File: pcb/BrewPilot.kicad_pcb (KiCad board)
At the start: 2 copper layers, 113 x 129 mm, 57 parts, among them J1 5V Power, J10 Boiler Probe, J11 SOL_L_FUSE, J12 5V_FUSE_5x20mm, J13 I2C Port, J2 Flow Meter Group One, J3 Flow Meter Group Two, J4 FlexGPIO_1, J5 FlexGPIO_2, J6 RelayOut_1, J7 RelayOut2, J8 Solenoid Power, J9 Pump Power, K1 G3MB-202P DC5, K2 G3MB-202P DC5, K3 G3MB-202P DC5, K4 G3MB-202P DC5, K5 G3MB-202P DC5, Q1 BC547, Q2 BC547, Q3 BC547, Q4 BC547, Q5 BC547, U1 esp32

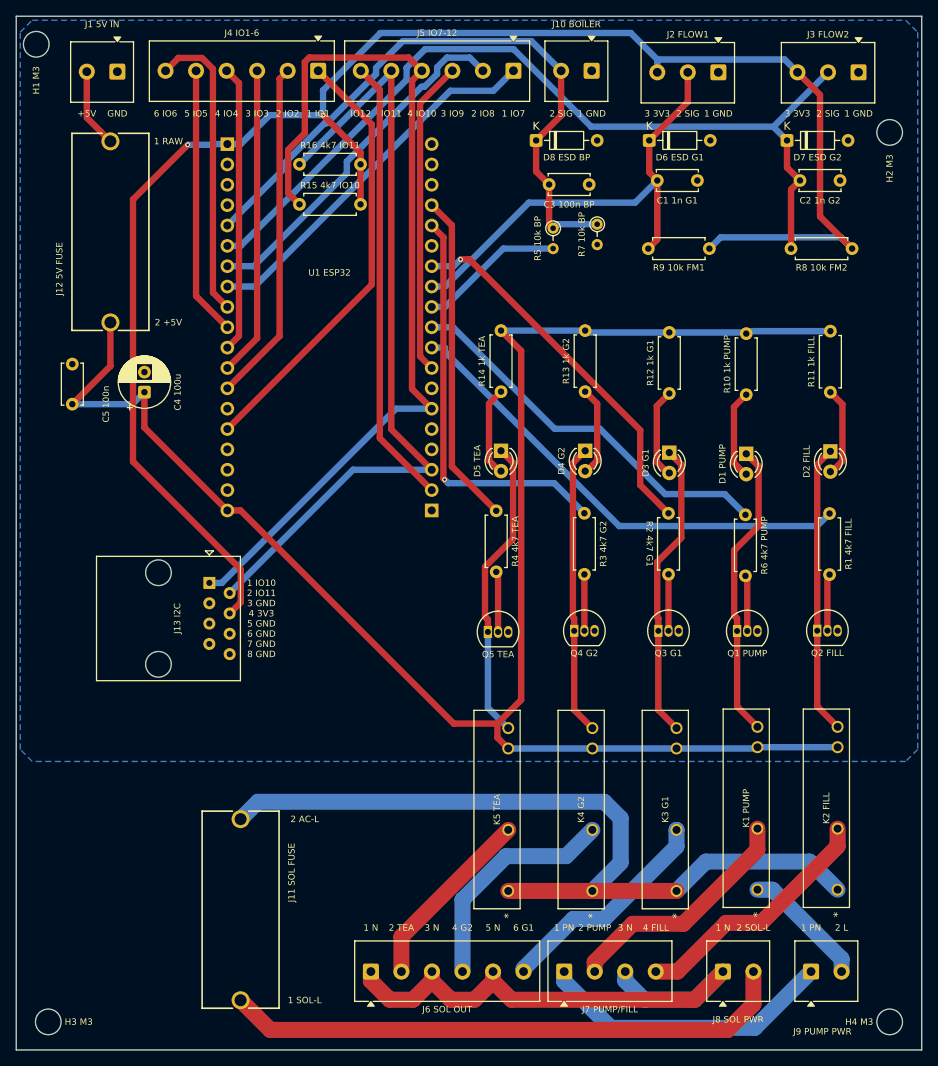
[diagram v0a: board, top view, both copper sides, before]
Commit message: made pcb layout more compact
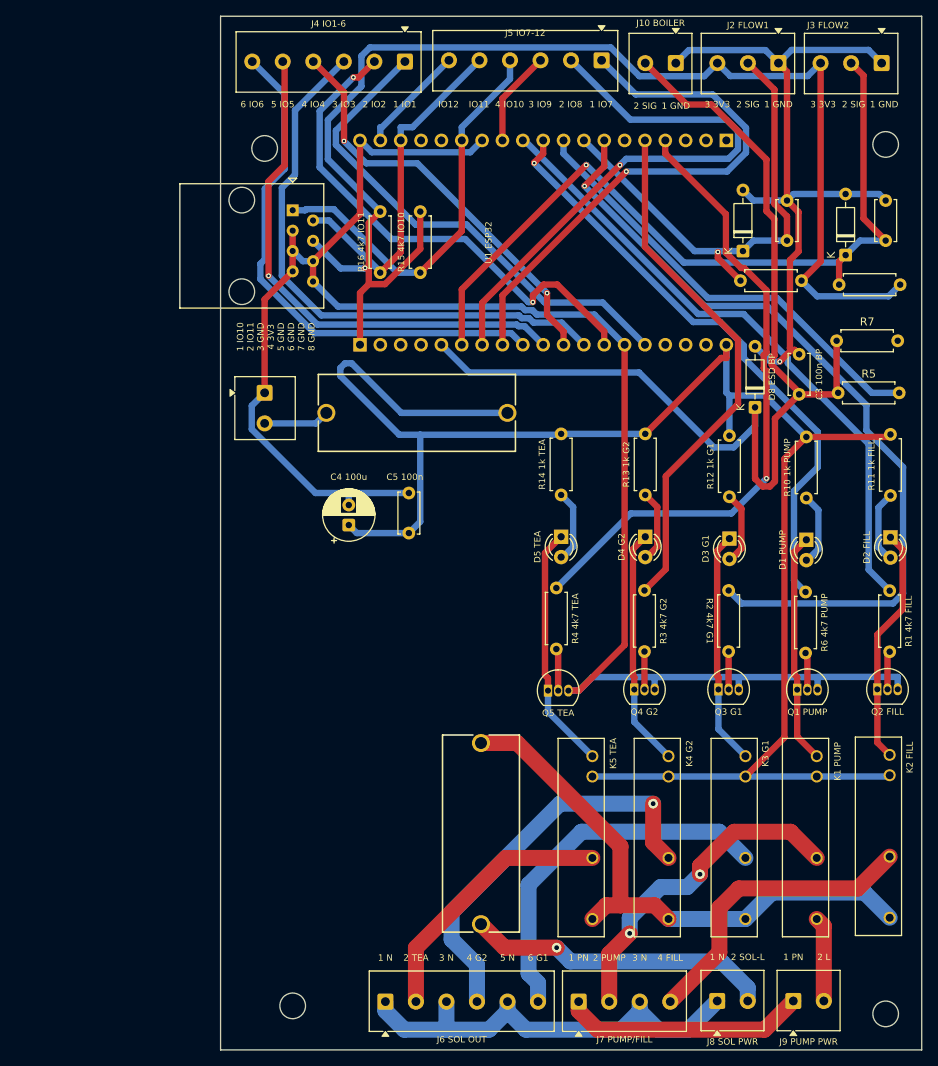
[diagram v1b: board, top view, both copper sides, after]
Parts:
- R5, R7: footprint Resistor_THT:R_Axial_DIN0204_L3.6mm_D1.6mm_P2.54mm_Vertical -> Resistor_THT:R_Axial_DIN0207_L6.3mm_D2.5mm_P7.62mm_Horizontal
- moved J13 47.6 mm to (151.5, 60.2)
- moved C5 45.0 mm to (166.0, 100.5)
- moved J12 44.4 mm to (167.0, 85.5), turned to 0 degrees
- moved J1 44.1 mm to (148.0, 83.0), turned to -90 degrees
- moved D8 43.1 mm to (209.2, 84.8), turned to 90 degrees
- moved R5 41.1 mm to (219.6, 83.0), turned to 0 degrees
- moved C3 40.7 mm to (214.7, 83.2), turned to 90 degrees
- moved R7 33.2 mm to (219.4, 76.5), turned to 0 degrees
- moved J11 31.5 mm to (175.0, 138.0)
- moved H1 31.3 mm to (148.0, 52.5)
- moved H3 30.6 mm to (151.5, 159.5)
- moved C4 30.4 mm to (158.5, 99.5)
- moved D6 18.1 mm to (207.7, 65.3), turned to 90 degrees
- moved C1 17.8 mm to (213.2, 64.0), turned to 90 degrees
- moved D7 16.1 mm to (220.5, 65.8), turned to 90 degrees
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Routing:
- net GND: track 0.00 -> 319.9 mm, vias 0 -> 1
- net FLEXIBLE_IO_10: track 115.2 -> 50.4 mm
- net FLEXIBLE_IO_11: track 99.9 -> 43.6 mm
- net CONTROL_RELAY_GROUP_ONE: track 47.0 -> 101.6 mm
- net IN_BOILER_PROBE: track 81.1 -> 134.9 mm
- net +3.3V: track 211.7 -> 165.9 mm, vias 2 -> 1
- net FLEXIBLE_IO_12: track 56.0 -> 13.7 mm
- net CONTROL_RELAY_TEA: track 41.5 -> 79.8 mm, vias 0 -> 1
- net OUT_BOILER_PROBE_VOLTAGE: track 18.2 -> 55.9 mm
- net SOL_L: track 70.9 -> 38.2 mm, vias 0 -> 1
- net FLEXIBLE_IO_03: track 38.6 -> 71.2 mm
- net AC_SOLENOID_PHASE: track 103.8 -> 71.3 mm
- net FLEXIBLE_IO_05: track 33.6 -> 65.5 mm, vias 0 -> 1
- net FLEXIBLE_IO_06: track 37.6 -> 66.2 mm
- net FLEXIBLE_IO_09: track 39.4 -> 12.0 mm
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- removed copper zone on B.Cu, net GND
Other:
- board size 113 x 129 mm -> 87.5 x 129 mm
- board text removed: "+5V"
- board text removed: "1 RAW"
- board text removed: "1 SOL-L"
- board text removed: "2 +5V"
- board text removed: "2 AC-L"
- board text removed: "C1 1n G1"
- board text removed: "C2 1n G2"
- board text removed: "D6 ESD G1"
- board text removed: "D7 ESD G2"
- board text removed: "GND"
- board text removed: "H1 M3"
- board text removed: "H2 M3"
- board text removed: "H3 M3"
- board text removed: "H4 M3"
- board text removed: "J1 5V IN"
- board text removed: "J11 SOL FUSE"
- board text removed: "J12 5V FUSE"
- board text removed: "J13 I2C"
- board text removed: "R5 10k BP"
- board text removed: "R7 10k BP"
- board text removed: "R8 10k FM2"
- board text removed: "R9 10k FM1"
